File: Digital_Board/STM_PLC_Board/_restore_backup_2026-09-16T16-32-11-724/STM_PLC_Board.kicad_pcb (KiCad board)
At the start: 2 copper layers, 99.5 x 80 mm, 70 parts, among them J1 JTAG_10CON_SWD, J2 Misc_STM32_Conn, J3 Conn_02x14_Odd_Even_Female, J4 JTAG_ST8500_CON, J5 3pin_61300311121, J6 ViperJACK, J7 Barrel_Jack_Switch, J8 USB2.0_Molex, Q1 2N7002, Q2 2N7002, Q3 2N7002, Q4 2N7002, SW1 SW_Push, SW2 SW_DIP_x01, SW3 SW_DIP_x01, SW4 SW_SPDT, U1 STM32F446RET6, U2 AMS1117-3.3, Y1 25MHz

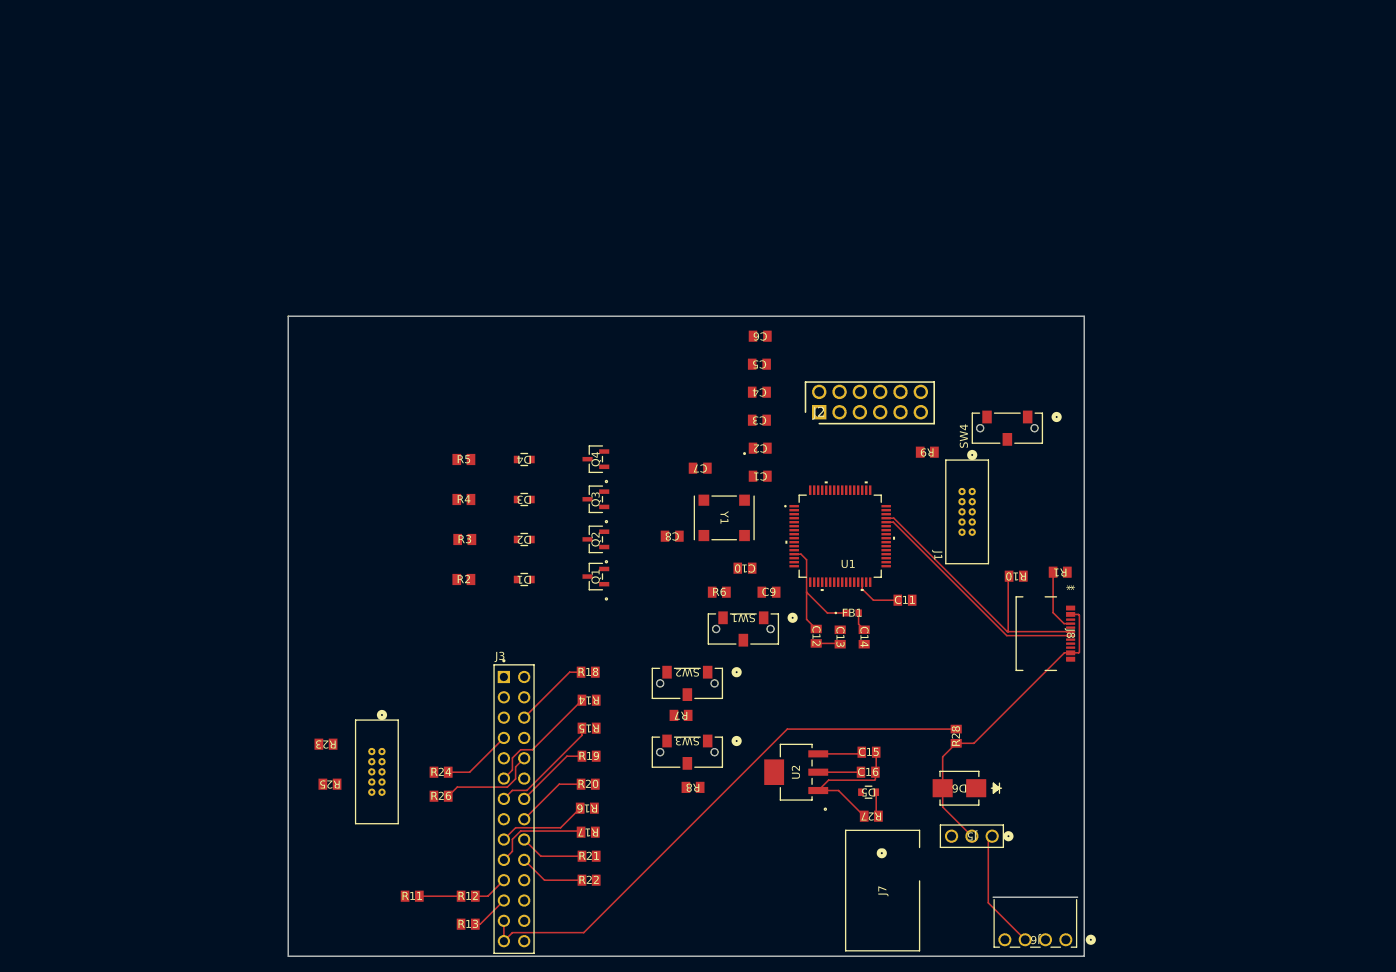
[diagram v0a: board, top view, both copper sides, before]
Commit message: pcb changes
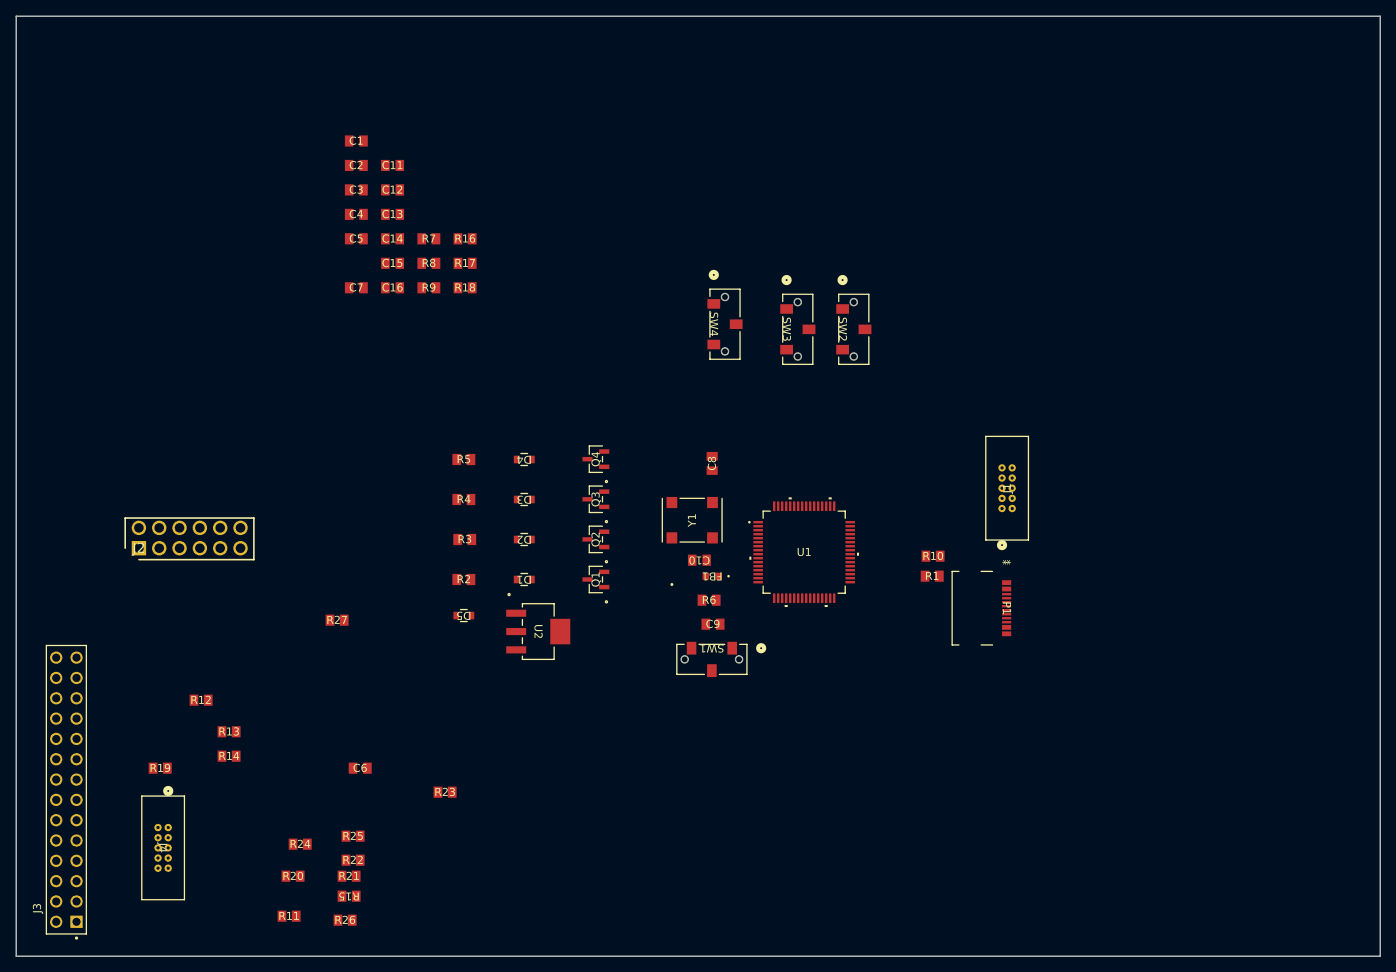
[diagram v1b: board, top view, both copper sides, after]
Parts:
- removed D6: SM6T18A, DigitalBoardLibrary:SMB_STM-M
- removed J5: 3pin_61300311121, DigitalBoardLibrary:3PIN_HEADER
- removed J6: ViperJACK, DigitalBoardLibrary:ViperJACK_0022152046
- removed J7: Barrel_Jack_Switch, DigitalBoardLibrary:jack_694106301002
- removed J8: USB2.0_Molex, DigitalBoardLibrary:USBC_2171790001_MOL
- removed R28: 0R, DigitalBoardLibrary:0805 SMD Resistor
- added P1: USB_C_Plug_USB2.0, DigitalBoardLibrary:USB_Molex_2.0, F.Cu at (222.0, 110.0)
- J1: value JTAG_10CON_SWD -> SHF-105-01-L-D-TH; footprint DigitalBoardLibrary:CONN10_SHF_12P7X5P08_SAI -> DigitalBoardLibrary:JTAG_CONN10_SHF_12P7X5P08_SAI
- J2: value Misc_STM32_Conn -> Conn_02x06_Odd_Even
- J4: value JTAG_ST8500_CON -> JTAG Connector; footprint DigitalBoardLibrary:CONN10_SHF_12P7X5P08_SAI -> DigitalBoardLibrary:JTAG_CONN10_SHF_12P7X5P08_SAI
- Y1: value 25MHz -> 24MHz
- moved J2 86.7 mm to (116.8, 102.5)
- moved C15 85.3 mm to (148.5, 66.9)
- moved C16 84.9 mm to (148.5, 69.9)
- moved C11 84.0 mm to (148.5, 54.7)
- moved C14 77.2 mm to (148.5, 63.8), turned to 0 degrees
- moved C13 76.9 mm to (148.5, 60.8), turned to 0 degrees
- moved C12 76.9 mm to (148.5, 57.7), turned to 0 degrees
- moved C6 73.6 mm to (144.5, 130.0), turned to 0 degrees
- moved R8 73.4 mm to (153.1, 66.9), turned to 0 degrees
- moved R16 72.8 mm to (157.6, 63.8), turned to 0 degrees
- moved R17 72.8 mm to (157.6, 66.9), turned to 0 degrees
- moved R27 71.1 mm to (141.6, 111.5), turned to 0 degrees
- moved R7 67.4 mm to (153.1, 63.8), turned to 0 degrees
- moved R9 65.6 mm to (153.1, 69.9), turned to 0 degrees
- moved C1 65.6 mm to (144.0, 51.6), turned to 0 degrees
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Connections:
- J3 pad 3: GND -> PLC_BOOT2
- J4 pad 10: unconnected-(J4-Pad10) -> GND
- J4 pad 2: PLC_JRST -> +3V3
- J4 pad 3: PLC_JTDI -> PLC_JRST
- J4 pad 4: PLC_JTMS -> GND
- J4 pad 5: PLC_JTCK -> PLC_JTDI
- J4 pad 6: unconnected-(J4-Pad6) -> GND
- J4 pad 7: PLC_JTDO -> PLC_JTMS
- J4 pad 8: Net-(J4-Pad8) -> GND
- J4 pad 9: unconnected-(J4-Pad9) -> PLC_JTCK
- R25 pad 2: Net-(J4-Pad8) -> Net-(J4-Pin_15)
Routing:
- net VDC_LD: track 70.1 -> 0.00 mm
- net VBUS: track 45.2 -> 0.00 mm
- net /STM_PLC_Board/USB_D+: track 36.0 -> 0.00 mm
- net /STM_PLC_Board/USB_D-: track 28.9 -> 0.00 mm
- net GND: track 21.3 -> 0.00 mm
- net +3.3VA: track 17.0 -> 0.00 mm
- net Net-(J6-Pin_3): track 15.1 -> 0.00 mm
- net Net-(J3-Pin_11): track 14.7 -> 0.00 mm
- net Net-(J3-Pin_13): track 13.9 -> 0.00 mm
- net PLC_JTDO: track 12.3 -> 0.00 mm
- net Net-(J3-Pin_19): track 12.1 -> 0.00 mm
- net Net-(J3-Pin_17): track 11.2 -> 0.00 mm
- net Net-(J3-Pin_6): track 9.46 -> 0.00 mm
- net Net-(J3-Pin_14): track 9.43 -> 0.00 mm
- net Net-(J3-Pin_16): track 8.93 -> 0.00 mm
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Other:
- board size 99.5 x 80 mm -> 170.5 x 117.5 mm
